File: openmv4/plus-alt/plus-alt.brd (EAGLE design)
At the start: 35.6 x 44.5 mm, 80 parts, among them M1 9774030243R, M2 9774030243R, Q1 BSS138, Q2 AO3401, U1 W25Q256JVEIQ_TR, U2 *, U3 ME6211C33M5G, U4 PAM2305AABADJ, U5 USBLC6-2, X1 MF-CON-MICROUSB-RIGHT, X2 USD-1040310811, X3 DF12-36-DS, X4 S2B-PH-K-S(LF)(SN), Y1 12M

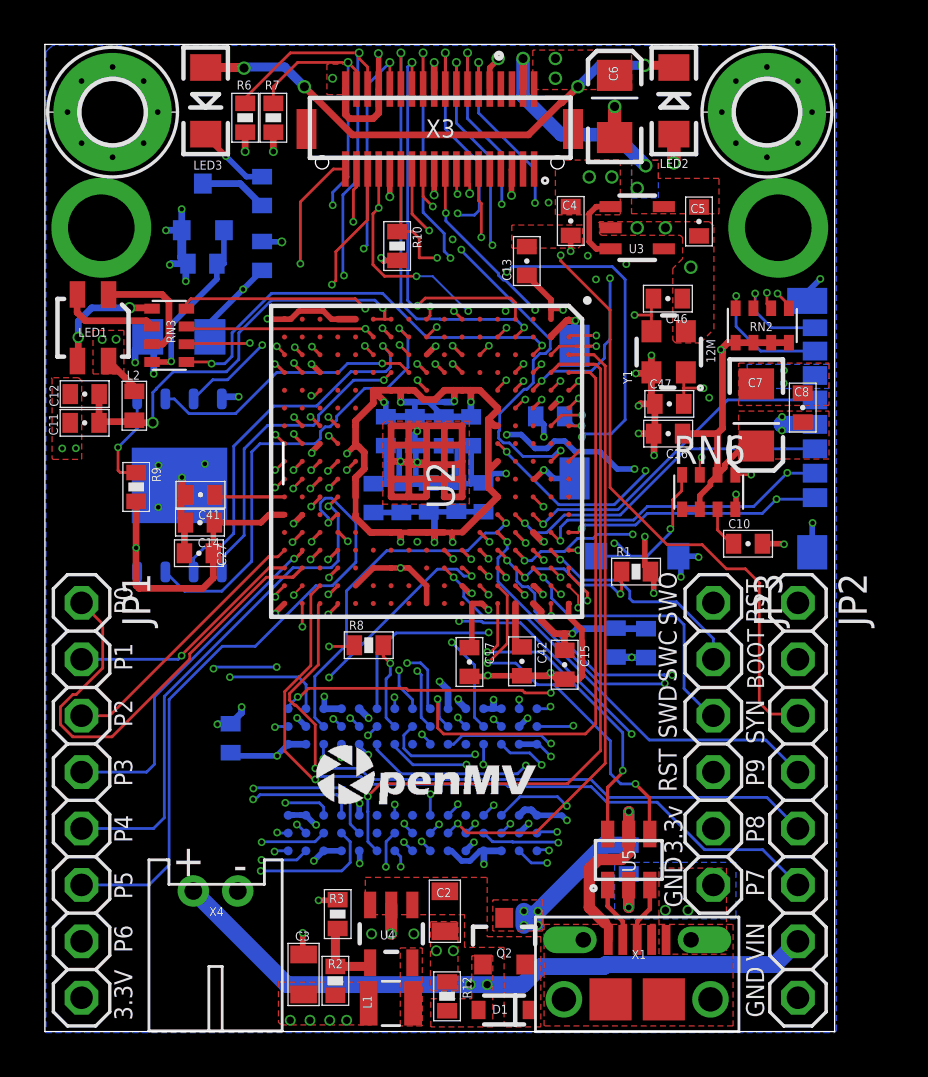
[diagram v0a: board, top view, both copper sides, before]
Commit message: Signals must be redone
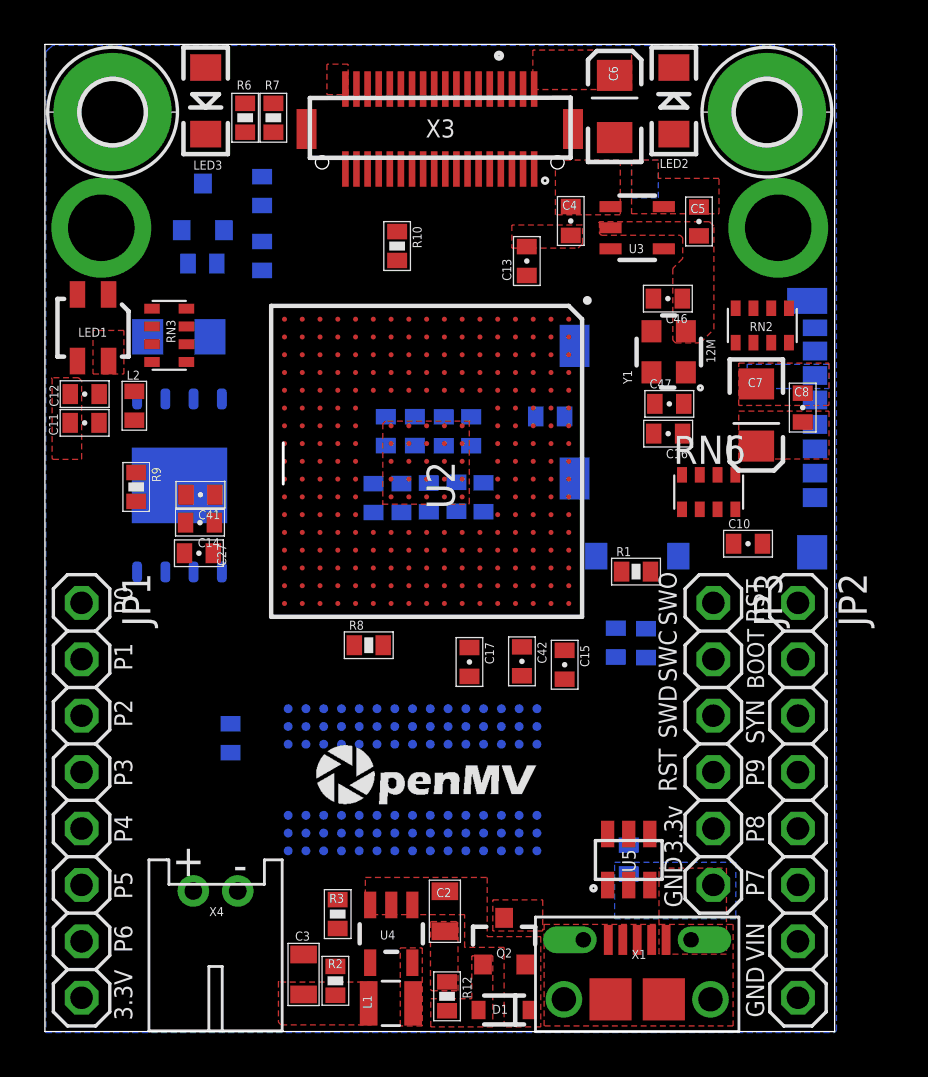
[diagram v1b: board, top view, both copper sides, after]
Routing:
- net GND: track 136.2 -> 0.00 mm, vias 77 -> 0
- net VCC: track 127.7 -> 0.00 mm, vias 48 -> 0
- net SPI3_SCLK/TRACESWO: track 40.2 -> 0.00 mm, vias 3 -> 0
- net VBUS: track 39.8 -> 0.00 mm, vias 9 -> 0
- net SDIO_D0: track 36.9 -> 0.00 mm, vias 3 -> 0
- net DCMI_FSIN: track 36.8 -> 0.00 mm, vias 2 -> 0
- net DRAM_CLKE: track 35.2 -> 0.00 mm, vias 2 -> 0
- net DAC: track 34.6 -> 0.00 mm, vias 1 -> 0
- net SDIO_D1: track 34.3 -> 0.00 mm, vias 3 -> 0
- net TIM4_CH1: track 33.8 -> 0.00 mm, vias 1 -> 0
- net DRAM_DQM1: track 33.6 -> 0.00 mm, vias 1 -> 0
- net DRAM_D29: track 32.5 -> 0.00 mm, vias 2 -> 0
- net DCMI_RST: track 32.4 -> 0.00 mm, vias 4 -> 0
- net DRAM_D28: track 32.3 -> 0.00 mm, vias 2 -> 0
- net I2C1_SCL: track 31.6 -> 0.00 mm, vias 3 -> 0
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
